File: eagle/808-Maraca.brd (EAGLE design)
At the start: 100 x 80 mm, 46 parts, among them IC1 TL071P, Q1 2N3904, Q2 2N3906, Q3 2N3906, Q4 2N3904, Q59 2N3904, Q60 2N3906

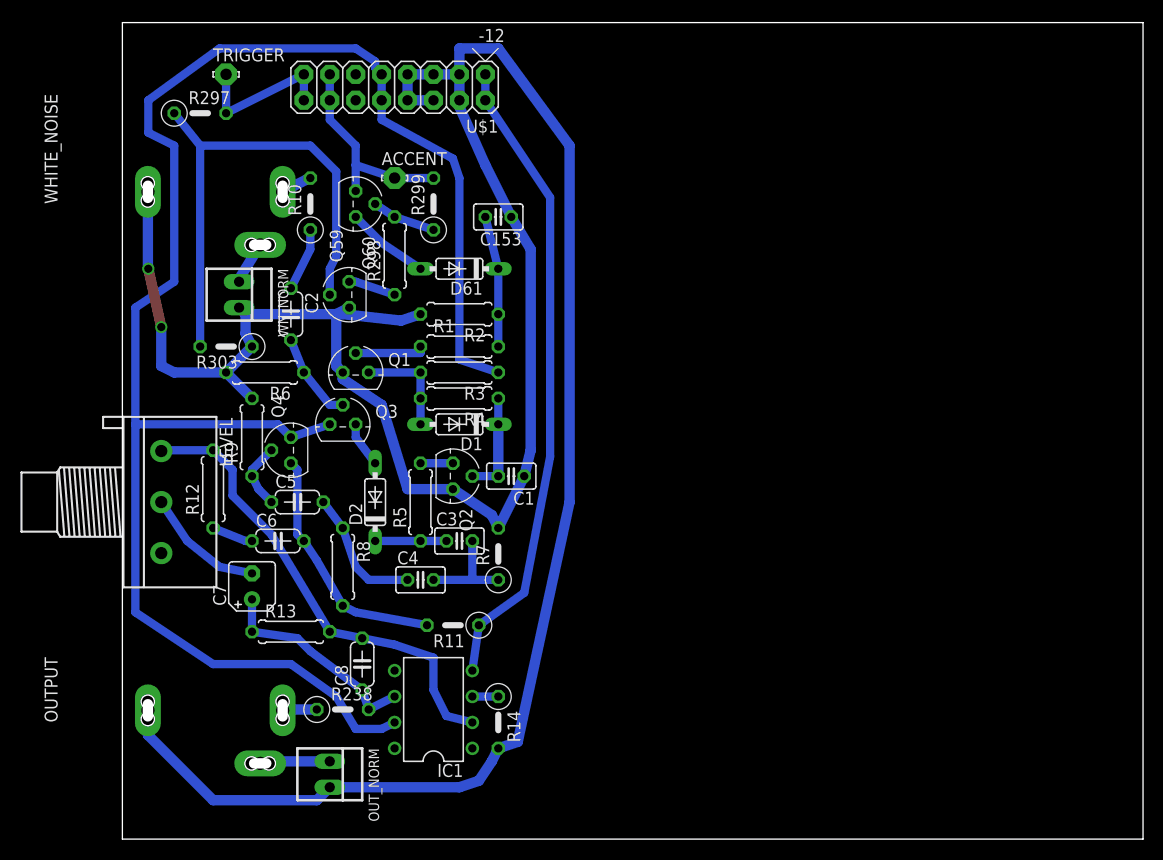
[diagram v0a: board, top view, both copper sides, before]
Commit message: cutout
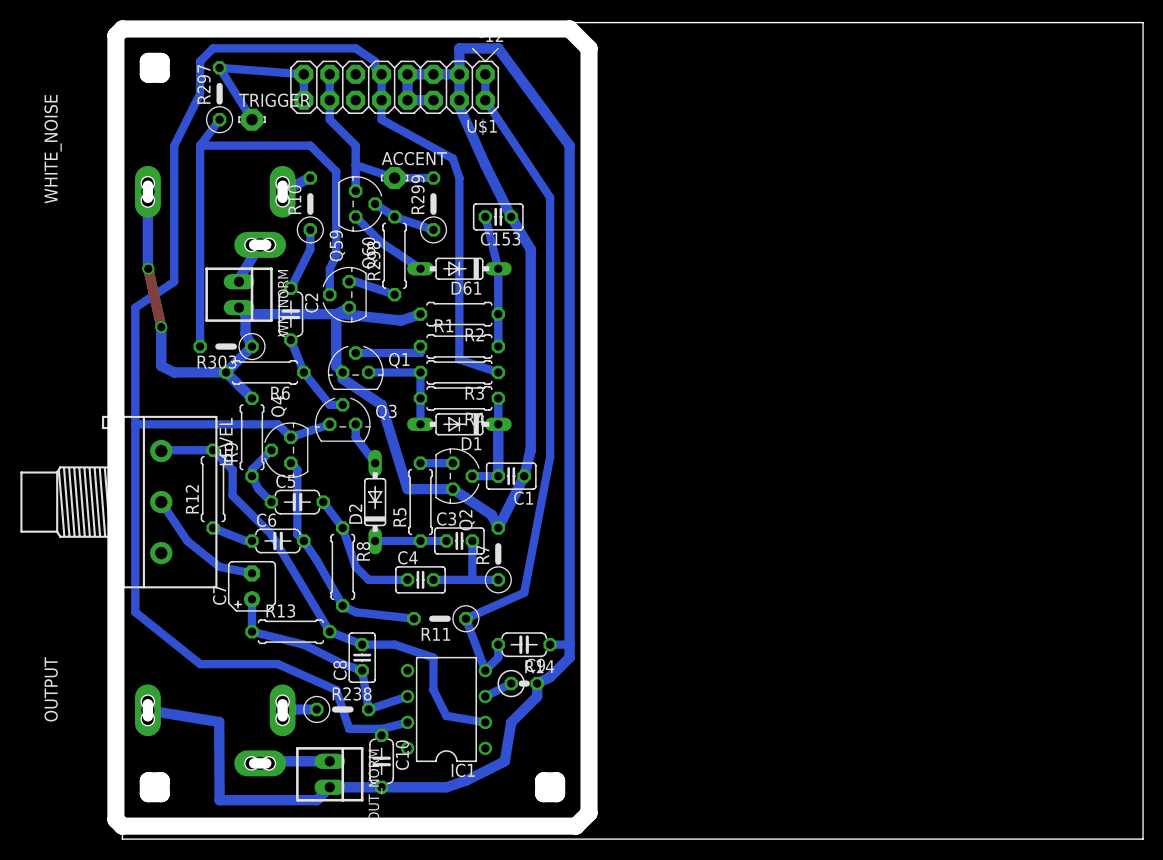
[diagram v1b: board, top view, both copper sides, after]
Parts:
- added C10, C9: 10n, TR808clone:C050-024X044
- C8: device TR808clone:C050-024X044 -> TR808clone:C025-025X050
- R14: device TR808clone:0207/5V -> TR808clone:0207/2V
- moved TRIGGER 5.12 mm to (12.7, 70.5)
- moved R14 4.58 mm to (39.4, 15.2), turned to 0 degrees
- moved R297 2.69 mm to (9.53, 73.0), turned to 90 degrees
- moved R11 1.42 mm to (31.1, 21.6)
- moved IC1 1.27 mm to (31.8, 12.7)
- moved C8 0.64 mm to (23.5, 17.8)
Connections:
- net +12V: now also C10.1
- net -12V: now also C9.2
- net GND: now also C10.2, C9.1
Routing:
- net GND: track 262.3 -> 268.1 mm
- net -12V: track 62.9 -> 67.7 mm
- net N$20: track 14.9 -> 16.8 mm
- net N$8: track 20.7 -> 22.6 mm
- net N$17: track 46.0 -> 47.4 mm
- net N$16: track 24.1 -> 22.7 mm
- net N$318: track 50.4 -> 49.5 mm
- net +12V: track 165.5 -> 164.6 mm
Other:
- board size 100 x 80 mm -> 100.6 x 80 mm
